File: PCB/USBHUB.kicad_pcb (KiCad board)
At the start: 2 copper layers, 67.4 x 49.4 mm, 33 parts, among them J1 USB_C_Receptacle_USB2.0_16P, J2 USB_C_Receptacle_USB2.0_16P, J3 USB_C_Receptacle_USB2.0_16P, J4 USB_A, J5 USB_A, Y1 12 mhz

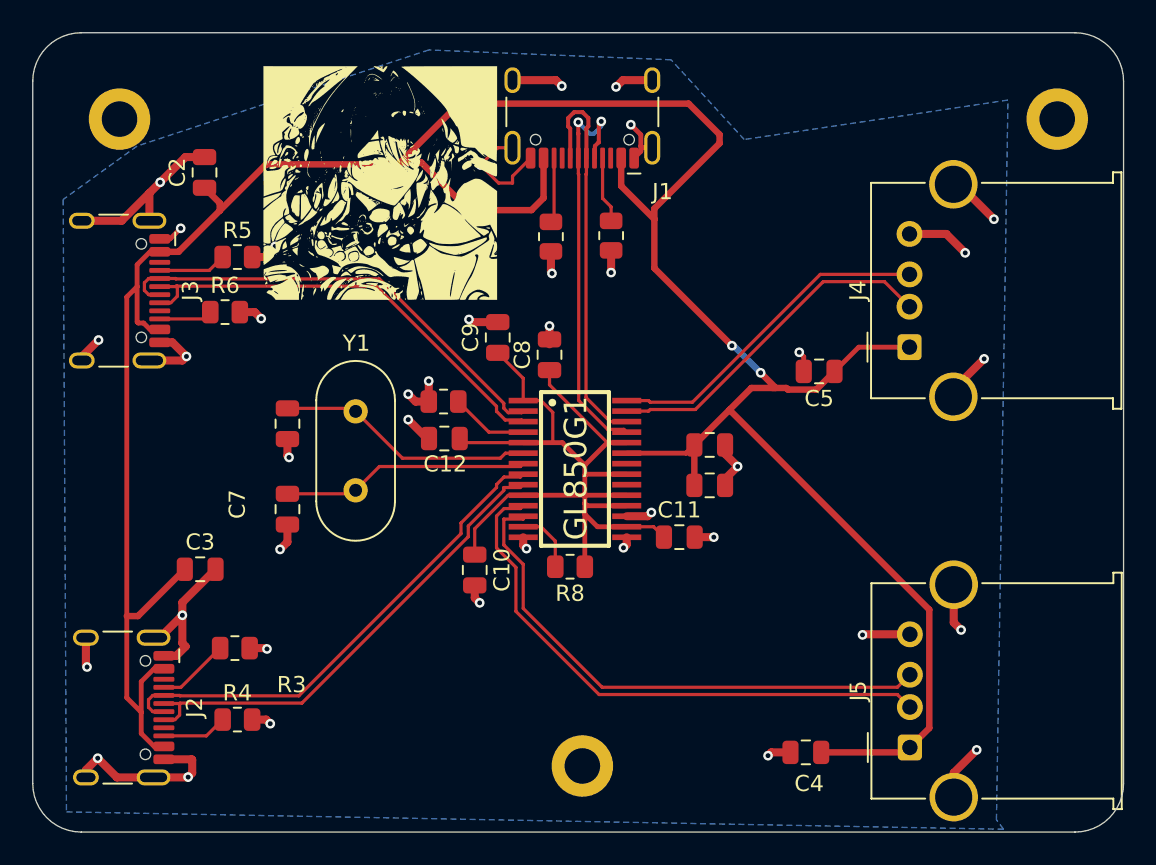
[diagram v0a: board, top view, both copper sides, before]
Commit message: PCB UPDATE
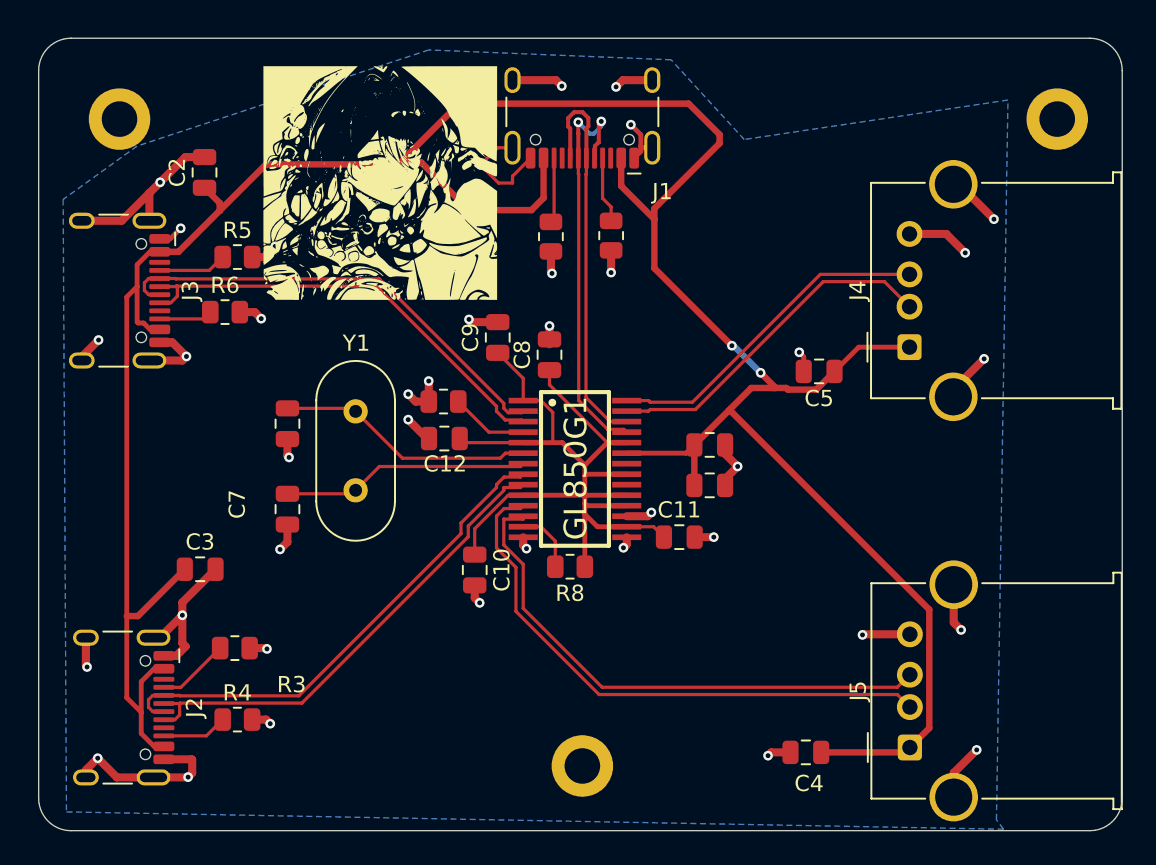
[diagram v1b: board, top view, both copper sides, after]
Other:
- board size 67.4 x 49.4 mm -> 67 x 49 mm
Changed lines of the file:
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@@
 		)
 		(embedded_fonts no)
+		(model "C:/Users/abhinav/Downloads/ssop-28-ic-case.snapshot.2/ssop28.stp"
+			(offset
+				(xyz -4.2 3.5 0)
+			)
+			(scale
+				(xyz 1 1 1)
+			)
+			(rotate
+				(xyz -0 -0 90)
+			)
+		)
 	)
 	(footprint "Capacitor_SMD:C_0805_2012Metric"
@@
 		(descr "HC-49/U, Crystal, http://5hertz.com/pdfs/04404_D.pdf")
 		(property "Reference" "Y1"
-			(at -4.2132 -0.0508 180)
+			(at -4.2132 -0.0508 0)
 			(layer "F.SilkS")
 			(effects
@@
 			)
 			(scale
-				(xyz 1 1 0.2)
+				(xyz 1 1 1)
 			)
 			(rotate
-				(xyz -0 -0 -0)
+				(xyz 0 0 0)
 			)
 		)
@@
 	)
 	(gr_arc
-		(start 119.634 79.660762)
-		(mid 120.51268 77.539442)
-		(end 122.634 76.660762)
+		(start 120 79)
+		(mid 120.585786 77.585786)
+		(end 122 77)
 		(stroke
 			(width 0.05)
@@
 	)
 	(gr_line
-		(start 119.634 123.0856)
-		(end 119.634 79.660762)
+		(start 120 124)
+		(end 120 79)
 		(stroke
 			(width 0.05)
@@
 	)
 	(gr_line
-		(start 122.634 76.660762)
-		(end 184.083469 76.660762)
+		(start 122 77)
+		(end 185 77)
 		(stroke
 			(width 0.05)
@@
 	)
 	(gr_arc
-		(start 122.634 126.0856)
-		(mid 120.51268 125.20692)
-		(end 119.634 123.0856)
+		(start 122 126)
+		(mid 120.585786 125.414214)
+		(end 120 124)
 		(stroke
 			(width 0.05)
@@
 	)
 	(gr_arc
-		(start 184.083469 76.660762)
-		(mid 186.204789 77.539442)
-		(end 187.083469 79.660762)
+		(start 185 77)
+		(mid 186.414214 77.585786)
+		(end 187 79)
 		(stroke
 			(width 0.05)
@@
 	)
 	(gr_line
-		(start 184.083469 126.0856)
-		(end 122.634 126.0856)
+		(start 185 126)
+		(end 122 126)
 		(stroke
 			(width 0.05)
@@
 	)
 	(gr_line
-		(start 187.083469 79.660762)
-		(end 187.083469 123.0856)
+		(start 187 79)
+		(end 187 124)
 		(stroke
 			(width 0.05)
@@
 	)
 	(gr_arc
-		(start 187.083469 123.0856)
-		(mid 186.204787 125.206909)
-		(end 184.083469 126.0856)
+		(start 187 124)
+		(mid 186.414214 125.414214)
+		(end 185 126)
 		(stroke
 			(width 0.05)
